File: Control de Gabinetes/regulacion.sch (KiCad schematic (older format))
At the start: 13 parts, among them J1 Conn_01x03_MountingPin, J3.3V 3.3V, J5V 5V, U2 LM1117-3.3, U3 LM1117-5.0

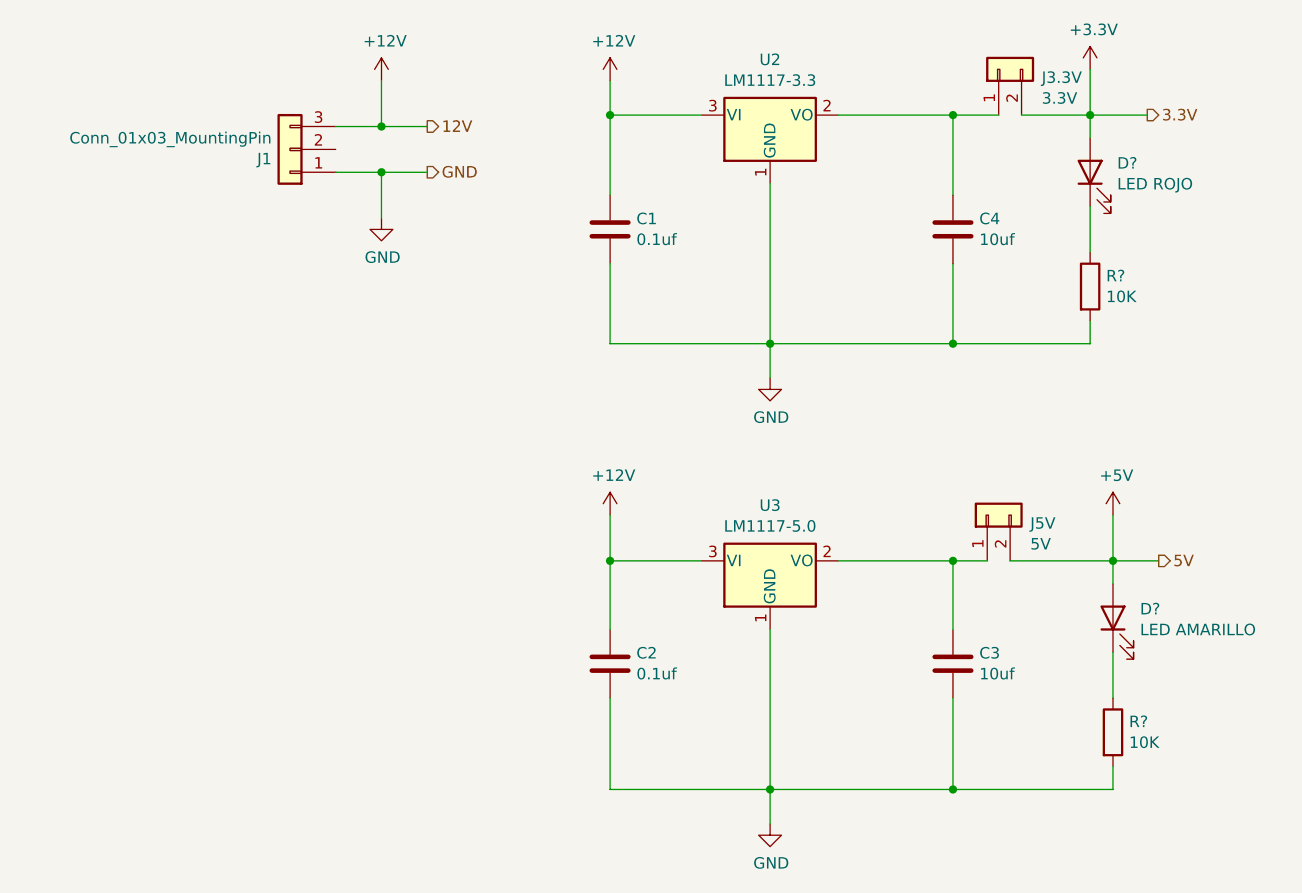
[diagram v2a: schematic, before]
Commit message: AVANCE 7/7/2021
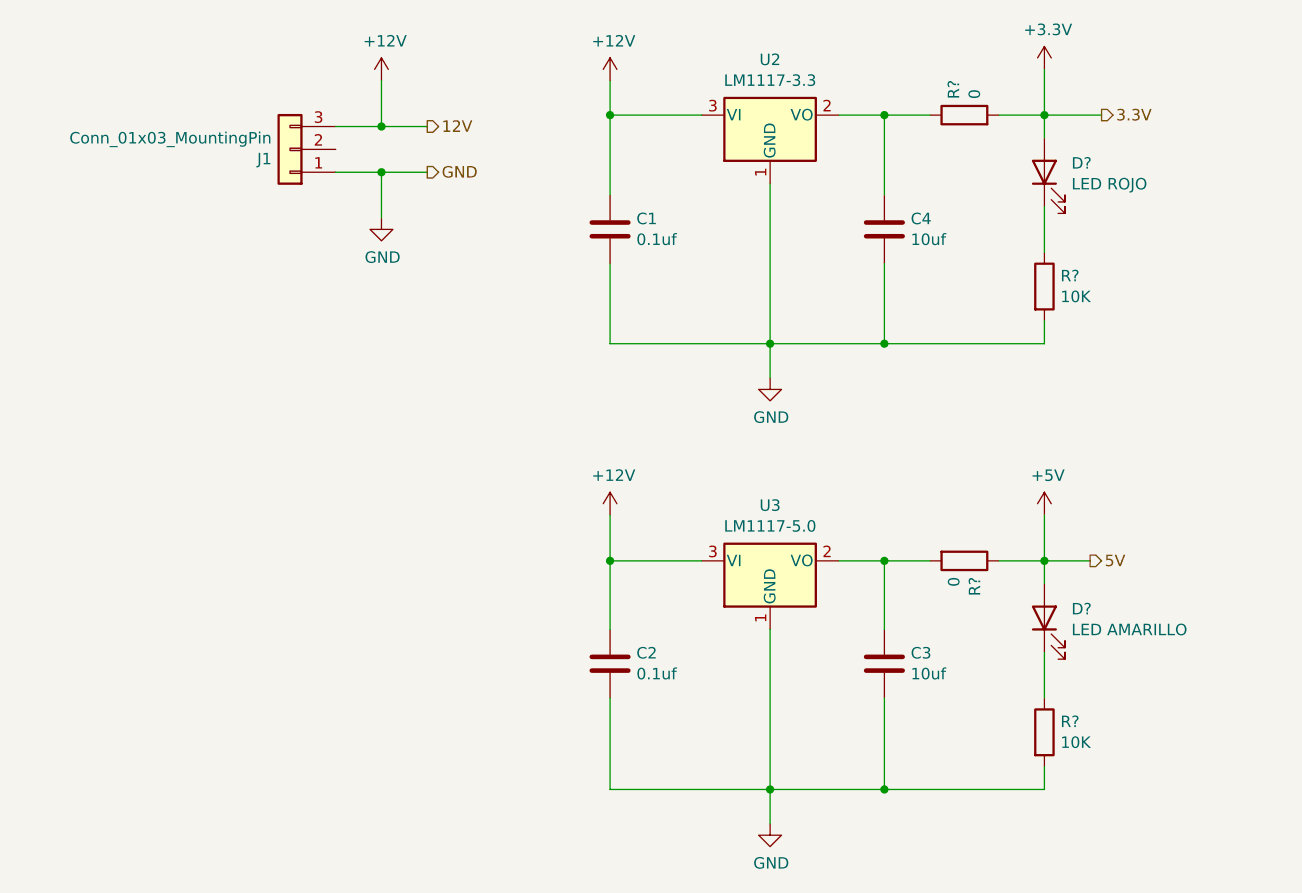
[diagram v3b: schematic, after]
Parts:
- removed J3.3V: 3.3V, Connector_PinHeader_2.54mm:PinHeader_1x02_P2.54mm_Vertical, symbol Connector_Generic:Conn_01x02
- removed J5V: 5V, Connector_PinHeader_2.54mm:PinHeader_1x02_P2.54mm_Vertical, symbol Connector_Generic:Conn_01x02
- added R? (x2): 0, Resistor_SMD:R_0805_2012Metric, symbol Device:R
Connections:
- net +3V3: now also R?.2
- net +5V: now also R?.1
- net at C4.1, U2.2 (VO): now also R?.1
- net at C3.1, U3.2 (VO): now also R?.2
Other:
- moved on the sheet: C3, C4, D?, R?
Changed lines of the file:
@@
 L power:+3.3V #PWR0106
 U 1 1 6098BC81
-P 5200 1150
-F 0 "#PWR0106" H 5200 1000 50  0001 C CNN
-F 1 "+3.3V" H 5215 1323 50  0000 C CNN
-F 2 "" H 5200 1150 50  0001 C CNN
-F 3 "" H 5200 1150 50  0001 C CNN
-	1    5200 1150
+P 5000 1150
+F 0 "#PWR0106" H 5000 1000 50  0001 C CNN
+F 1 "+3.3V" H 5015 1323 50  0000 C CNN
+F 2 "" H 5000 1150 50  0001 C CNN
+F 3 "" H 5000 1150 50  0001 C CNN
+	1    5000 1150
 	1    0    0    -1
 $EndComp
@@
 L Device:C C4
 U 1 1 60997875
-P 4600 1850
-F 0 "C4" H 4715 1896 50  0000 L CNN
-F 1 "10uf" H 4715 1805 50  0000 L CNN
-F 2 "Capacitor_SMD:C_0805_2012Metric" H 4638 1700 50  0001 C CNN
-F 3 "~" H 4600 1850 50  0001 C CNN
-	1    4600 1850
+P 4300 1850
+F 0 "C4" H 4415 1896 50  0000 L CNN
+F 1 "10uf" H 4415 1805 50  0000 L CNN
+F 2 "Capacitor_SMD:C_0805_2012Metric" H 4338 1700 50  0001 C CNN
+F 3 "~" H 4300 1850 50  0001 C CNN
+	1    4300 1850
 	1    0    0    -1
 $EndComp
@@
 	1    0    0    -1
 $EndComp
-Text HLabel 5450 1350 2    50   Output ~ 0
+Text HLabel 5250 1350 2    50   Output ~ 0
 3.3V
 Wire Wire Line
-	5200 1350 5450 1350
-Text HLabel 5500 3300 2    50   Output ~ 0
+	5000 1350 5250 1350
+Text HLabel 5200 3300 2    50   Output ~ 0
 5V
 Wire Wire Line
-	5300 3300 5500 3300
+	5000 3300 5200 3300
 $Comp
 L power:+5V #PWR0111
 U 1 1 6099CBA4
-P 5300 3100
-F 0 "#PWR0111" H 5300 2950 50  0001 C CNN
-F 1 "+5V" H 5315 3273 50  0000 C CNN
-F 2 "" H 5300 3100 50  0001 C CNN
-F 3 "" H 5300 3100 50  0001 C CNN
-	1    5300 3100
+P 5000 3100
+F 0 "#PWR0111" H 5000 2950 50  0001 C CNN
+F 1 "+5V" H 5015 3273 50  0000 C CNN
+F 2 "" H 5000 3100 50  0001 C CNN
+F 3 "" H 5000 3100 50  0001 C CNN
+	1    5000 3100
 	1    0    0    -1
 $EndComp
@@
 L Device:LED D?
 U 1 1 60E20F7B
-P 5200 1600
-F 0 "D?" V 5239 1482 50  0000 R CNN
-F 1 "LED ROJO" V 5148 1482 50  0000 R CNN
-F 2 "LED_SMD:LED_0805_2012Metric" H 5200 1600 50  0001 C CNN
-F 3 "~" H 5200 1600 50  0001 C CNN
-	1    5200 1600
+P 5000 1600
+F 0 "D?" V 5039 1482 50  0000 R CNN
+F 1 "LED ROJO" V 4948 1482 50  0000 R CNN
+F 2 "LED_SMD:LED_0805_2012Metric" H 5000 1600 50  0001 C CNN
+F 3 "~" H 5000 1600 50  0001 C CNN
+	1    5000 1600
 	0    -1   -1   0
 $EndComp
@@
 L Device:R R?
 U 1 1 60E239E3
-P 5200 2100
-F 0 "R?" H 5270 2146 50  0000 L CNN
-F 1 "10K" H 5270 2055 50  0000 L CNN
-F 2 "Resistor_SMD:R_0805_2012Metric" V 5130 2100 50  0001 C CNN
-F 3 "~" H 5200 2100 50  0001 C CNN
-	1    5200 2100
-	1    0    0    -1
-$EndComp
-Wire Wire Line
-	4600 1350 4600 1700
+P 5000 2100
+F 0 "R?" H 5070 2146 50  0000 L CNN
+F 1 "10K" H 5070 2055 50  0000 L CNN
+F 2 "Resistor_SMD:R_0805_2012Metric" V 4930 2100 50  0001 C CNN
+F 3 "~" H 5000 2100 50  0001 C CNN
+	1    5000 2100
+	1    0    0    -1
+$EndComp
+Wire Wire Line
+	4300 1350 4300 1700
 Wire Wire Line
 	3100 1350 3100 1700
 Wire Wire Line
-	5200 1750 5200 1950
-Wire Wire Line
-	5200 1450 5200 1350
-Connection ~ 5200 1350
+	5000 1750 5000 1950
+Wire Wire Line
+	5000 1450 5000 1350
+Connection ~ 5000 1350
 $Comp
 L Device:LED D?
 U 1 1 60E29EA4
-P 5300 3550
-F 0 "D?" V 5339 3432 50  0000 R CNN
-F 1 "LED AMARILLO" V 5248 3432 50  0000 R CNN
-F 2 "LED_SMD:LED_0805_2012Metric" H 5300 3550 50  0001 C CNN
-F 3 "~" H 5300 3550 50  0001 C CNN
-	1    5300 3550
+P 5000 3550
+F 0 "D?" V 5039 3432 50  0000 R CNN
+F 1 "LED AMARILLO" V 4948 3432 50  0000 R CNN
+F 2 "LED_SMD:LED_0805_2012Metric" H 5000 3550 50  0001 C CNN
+F 3 "~" H 5000 3550 50  0001 C CNN
+	1    5000 3550
 	0    -1   -1   0
 $EndComp
@@
 L Device:R R?
 U 1 1 60E2A004
-P 5300 4050
-F 0 "R?" H 5370 4096 50  0000 L CNN
-F 1 "10K" H 5370 4005 50  0000 L CNN
-F 2 "Resistor_SMD:R_0805_2012Metric" V 5230 4050 50  0001 C CNN
-F 3 "~" H 5300 4050 50  0001 C CNN
-	1    5300 4050
-	1    0    0    -1
-$EndComp
-Wire Wire Line
-	5300 3700 5300 3900
+P 5000 4050
+F 0 "R?" H 5070 4096 50  0000 L CNN
+F 1 "10K" H 5070 4005 50  0000 L CNN
+F 2 "Resistor_SMD:R_0805_2012Metric" V 4930 4050 50  0001 C CNN
+F 3 "~" H 5000 4050 50  0001 C CNN
+	1    5000 4050
+	1    0    0    -1
+$EndComp
+Wire Wire Line
+	5000 3700 5000 3900
 $Comp
 L Device:C C3
 U 1 1 60999295
-P 4600 3750
-F 0 "C3" H 4715 3796 50  0000 L CNN
-F 1 "10uf" H 4715 3705 50  0000 L CNN
-F 2 "Capacitor_SMD:C_0805_2012Metric" H 4638 3600 50  0001 C CNN
-F 3 "~" H 4600 3750 50  0001 C CNN
-	1    4600 3750
-	1    0    0    -1
-$EndComp
-Wire Wire Line
-	5200 2250 5200 2350
-Wire Wire Line
-	5200 2350 4600 2350
+P 4300 3750
+F 0 "C3" H 4415 3796 50  0000 L CNN
+F 1 "10uf" H 4415 3705 50  0000 L CNN
+F 2 "Capacitor_SMD:C_0805_2012Metric" H 4338 3600 50  0001 C CNN
+F 3 "~" H 4300 3750 50  0001 C CNN
+	1    4300 3750
+	1    0    0    -1
+$EndComp
+Wire Wire Line
+	5000 2250 5000 2350
 Wire Wire Line
 	3100 2000 3100 2350
 Wire Wire Line
-	5300 4200 5300 4300
-Wire Wire Line
-	5300 4300 4600 4300
+	5000 4200 5000 4300
 Wire Wire Line
 	3100 4300 3100 3900
@@
 Connection ~ 3100 3300
 Wire Wire Line
-	4600 3300 4600 3600
-Wire Wire Line
-	4600 3900 4600 4300
-Connection ~ 4600 4300
-Wire Wire Line
-	5300 3400 5300 3300
-Connection ~ 5300 3300
+	4300 3300 4300 3600
+Wire Wire Line
+	4300 3900 4300 4300
+Wire Wire Line
+	5000 3400 5000 3300
+Connection ~ 5000 3300
 Wire Wire Line
 	3800 1650 3800 2350
@@
 Wire Wire Line
 	3800 4450 3800 4300
-$Comp
-L Connector_Generic:Conn_01x02 J3.3V
-U 1 1 60E4AE87
-P 4800 1150
-F 0 "J3.3V" V 4764 962 50  0000 R CNN
-F 1 "3.3V" V 4673 962 50  0000 R CNN
-F 2 "Connector_PinHeader_2.54mm:PinHeader_1x02_P2.54mm_Vertical" H 4800 1150 50  0001 C CNN
-F 3 "~" H 4800 1150 50  0001 C CNN
-	1    4800 1150
+Wire Wire Line
+	4300 2000 4300 2350
+Wire Wire Line
+	5000 1150 5000 1350
+Wire Wire Line
+	5000 3100 5000 3300
+Wire Wire Line
+	3800 4300 4300 4300
+Wire Wire Line
+	4100 3300 4300 3300
+Wire Wire Line
+	4100 1350 4300 1350
+$Comp
+L Device:R R?
+U 1 1 60E68AB2
+P 4650 1350
+F 0 "R?" H 4720 1396 50  0000 L CNN
+F 1 "0" H 4720 1305 50  0000 L CNN
+F 2 "Resistor_SMD:R_0805_2012Metric" V 4580 1350 50  0001 C CNN
+F 3 "~" H 4650 1350 50  0001 C CNN
+	1    4650 1350
 	0    -1   -1   0
 $EndComp
 Wire Wire Line
-	4600 2000 4600 2350
-Connection ~ 4600 2350
-Wire Wire Line
-	4600 2350 3800 2350
-Wire Wire Line
-	5200 1150 5200 1350
-Wire Wire Line
-	5300 3100 5300 3300
-$Comp
-L Connector_Generic:Conn_01x02 J5V
-U 1 1 60E51F0A
-P 4750 3100
-F 0 "J5V" V 4714 2912 50  0000 R CNN
-F 1 "5V" V 4623 2912 50  0000 R CNN
-F 2 "Connector_PinHeader_2.54mm:PinHeader_1x02_P2.54mm_Vertical" H 4750 3100 50  0001 C CNN
-F 3 "~" H 4750 3100 50  0001 C CNN
-F 4 "" V 4750 3100 50  0001 C CNN "Field4"
-	1    4750 3100
-	0    -1   -1   0
-$EndComp
-Wire Wire Line
-	3800 4300 4600 4300
-Wire Wire Line
-	4100 3300 4600 3300
-Wire Wire Line
-	4750 3300 4600 3300
-Connection ~ 4600 3300
-Wire Wire Line
-	4850 3300 5300 3300
-Wire Wire Line
-	4800 1350 4600 1350
-Wire Wire Line
-	4100 1350 4600 1350
-Connection ~ 4600 1350
-Wire Wire Line
-	4900 1350 5200 1350
+	4300 2350 3800 2350
+Wire Wire Line
+	4500 1350 4300 1350
+Connection ~ 4300 1350
+$Comp
+L Device:R R?
+U 1 1 60E7383A
+P 4650 3300
+F 0 "R?" H 4720 3346 50  0000 L CNN
+F 1 "0" H 4720 3255 50  0000 L CNN
+F 2 "Resistor_SMD:R_0805_2012Metric" V 4580 3300 50  0001 C CNN
+F 3 "~" H 4650 3300 50  0001 C CNN
+	1    4650 3300
+	0    1    1    0
+$EndComp
+Wire Wire Line
+	4800 1350 5000 1350
+Wire Wire Line
+	5000 2350 4300 2350
+Connection ~ 4300 2350
+Wire Wire Line
+	4800 3300 5000 3300
+Wire Wire Line
+	4500 3300 4300 3300
+Connection ~ 4300 3300
+Wire Wire Line
+	5000 4300 4300 4300
+Connection ~ 4300 4300
 $EndSCHEMATC
